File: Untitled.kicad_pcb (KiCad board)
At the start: 2 copper layers, 111.8 x 37.5 mm, 28 parts, among them J1 JAMMA, J2 CONN_01X06, J5 PWR_IN, J6 DC2DC, J7 SCART-F, SW1 SW_Push, SW2 SW_Push, SW3 SW_Push, U1 LD1117S33TR, U2 ESP32-WROOM, U3 TLC5926IDW, U4 TLC5926IDW

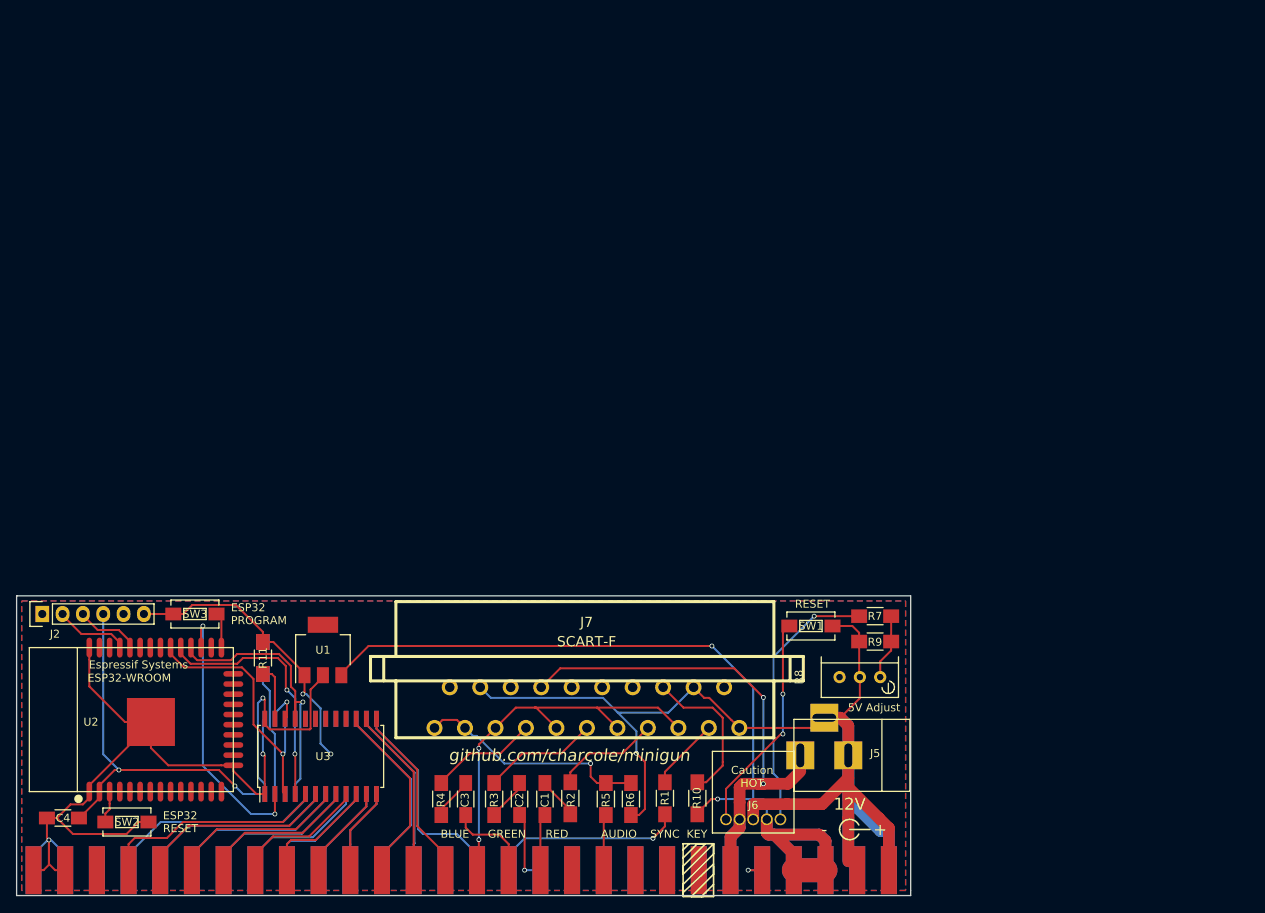
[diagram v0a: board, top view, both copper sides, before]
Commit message: Lynn almost done
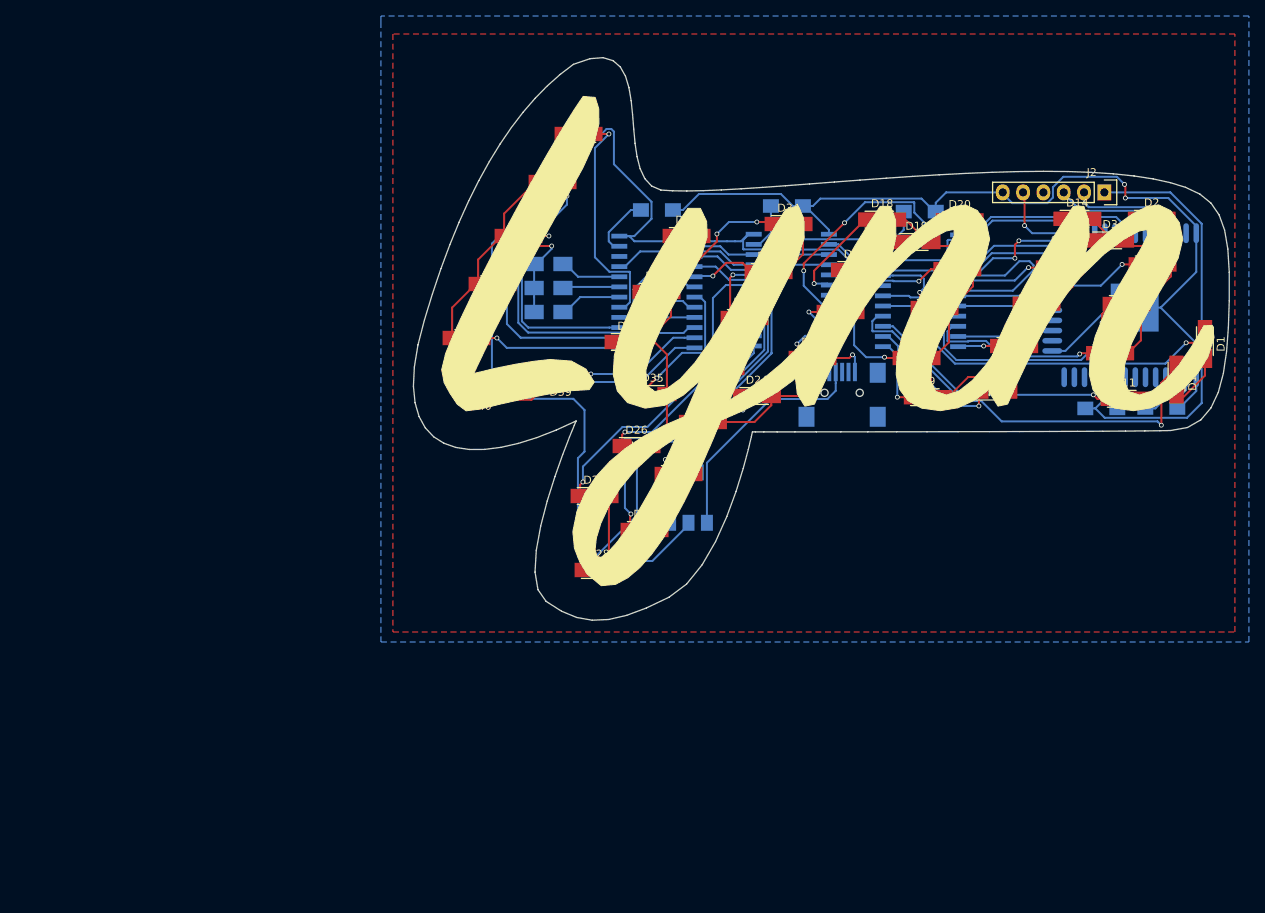
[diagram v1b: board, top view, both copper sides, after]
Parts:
- removed C1, C2, C3: 4.7u, Capacitors_SMD:C_1206_HandSoldering
- removed J5: PWR_IN, Connectors:BARREL_JACK
- removed J6: DC2DC, NQR010A0X4Z:NQR010A0X4Z
- removed J7: SCART-F, w_conn_av:SCART
- removed R10: 100, Resistors_SMD:R_1206_HandSoldering
- removed R3, R4: 330, Resistors_SMD:R_1206_HandSoldering
- removed R5: 10K, Resistors_SMD:R_1206_HandSoldering
- removed R6: 1K, Resistors_SMD:R_1206_HandSoldering
- removed R7: 240, Resistors_SMD:R_1206_HandSoldering
- removed R8: 500, Potentiometers:Potentiometer_Bourns_3296W_3-8Zoll_Inline_ScrewUp
- removed R9: 33, Resistors_SMD:R_1206_HandSoldering
- removed SW1, SW2, SW3: SW_Push, Buttons_Switches_SMD:SW_SPST_EVQPE1
- added D1: LED, LEDs:LED_1206_HandSoldering, F.Cu at (241.2, 94.2)
- added D10: LED, LEDs:LED_1206_HandSoldering, F.Cu at (214.8, 100.2)
- added D11: LED, LEDs:LED_1206_HandSoldering, F.Cu at (231.2, 101.1)
- added D12: LED, LEDs:LED_1206_HandSoldering, F.Cu at (237.7, 98.7)
- added D13: LED, LEDs:LED_1206_HandSoldering, F.Cu at (223.1, 84.7)
- added D14: LED, LEDs:LED_1206_HandSoldering, F.Cu at (225.3, 78.6)
- added D15: LED, LEDs:LED_1206_HandSoldering, F.Cu at (205.2, 96.0)
- added D16: LED, LEDs:LED_1206_HandSoldering, F.Cu at (207.4, 89.8)
- added D17: LED, LEDs:LED_1206_HandSoldering, F.Cu at (197.5, 85.0)
- added D18: LED, LEDs:LED_1206_HandSoldering, F.Cu at (200.9, 78.7)
- added D19: LED, LEDs:LED_1206_HandSoldering, F.Cu at (205.2, 81.5)
- added D2: LED, LEDs:LED_1206_HandSoldering, F.Cu at (234.6, 78.6)
- added D20: LED, LEDs:LED_1206_HandSoldering, F.Cu at (210.6, 78.8)
- added D21: LED, LEDs:LED_1206_HandSoldering, F.Cu at (210.3, 84.9)
- added D22: LED, LEDs:LED_1206_HandSoldering, F.Cu at (195.7, 90.2)
- added D23: LED, LEDs:LED_1206_HandSoldering, F.Cu at (192.2, 96.0)
- added D24: LED, LEDs:LED_1206_HandSoldering, F.Cu at (185.2, 100.8)
- added D25: LED, LEDs:LED_1206_HandSoldering, F.Cu at (178.5, 104.0)
- added D26: LED, LEDs:LED_1206_HandSoldering, F.Cu at (170.2, 107.0)
- added D27: LED, LEDs:LED_1206_HandSoldering, F.Cu at (164.9, 113.2)
- added D28: LED, LEDs:LED_1206_HandSoldering, F.Cu at (165.4, 122.5)
- added D29: LED, LEDs:LED_1206_HandSoldering, F.Cu at (171.2, 117.5)
- added D3: LED, LEDs:LED_1206_HandSoldering, F.Cu at (229.4, 81.3)
- added D30: LED, LEDs:LED_1206_HandSoldering, F.Cu at (175.4, 110.5)
- added D31: LED, LEDs:LED_1206_HandSoldering, F.Cu at (180.7, 97.2)
- added D32: LED, LEDs:LED_1206_HandSoldering, F.Cu at (183.7, 91.0)
- added D33: LED, LEDs:LED_1206_HandSoldering, F.Cu at (186.7, 85.2)
- added D34: LED, LEDs:LED_1206_HandSoldering, F.Cu at (189.2, 79.2)
- added D35: LED, LEDs:LED_1206_HandSoldering, F.Cu at (172.2, 100.5)
- added D36: LED, LEDs:LED_1206_HandSoldering, F.Cu at (169.2, 94.0)
- added D37: LED, LEDs:LED_1206_HandSoldering, F.Cu at (172.7, 87.8)
- added D38: LED, LEDs:LED_1206_HandSoldering, F.Cu at (176.4, 80.8)
- added D39: LED, LEDs:LED_1206_HandSoldering, F.Cu at (160.7, 98.2)
- added D4: LED, LEDs:LED_1206_HandSoldering, F.Cu at (234.7, 84.3)
- added D40: LED, LEDs:LED_1206_HandSoldering, F.Cu at (150.7, 100.0)
- added D41: LED, LEDs:LED_1206_HandSoldering, F.Cu at (148.9, 93.5)
- added D42: LED, LEDs:LED_1206_HandSoldering, F.Cu at (152.2, 86.8)
- added D43: LED, LEDs:LED_1206_HandSoldering, F.Cu at (155.4, 80.8)
- added D44: LED, LEDs:LED_1206_HandSoldering, F.Cu at (159.7, 74.0)
- added D45: LED, LEDs:LED_1206_HandSoldering, F.Cu at (162.9, 68.0)
- added D46: LED, LEDs:LED_1206_HandSoldering, B.Cu at (159.2, 90.2)
- added D47: LED, LEDs:LED_1206_HandSoldering, B.Cu at (159.2, 87.2)
- added D48: LED, LEDs:LED_1206_HandSoldering, B.Cu at (159.2, 84.2)
- added D5: LED, LEDs:LED_1206_HandSoldering, F.Cu at (231.4, 89.2)
- added D6: LED, LEDs:LED_1206_HandSoldering, F.Cu at (229.4, 95.4)
- added D7: LED, LEDs:LED_1206_HandSoldering, F.Cu at (220.2, 89.2)
- added D8: LED, LEDs:LED_1206_HandSoldering, F.Cu at (217.4, 94.5)
- added D9: LED, LEDs:LED_1206_HandSoldering, F.Cu at (206.6, 100.9)
- added U5: TLC5926IDW, Housings_SOIC:SOIC-24W_7.5x15.4mm_Pitch1.27mm, B.Cu at (172.8, 87.8)
- added lynn_outline: G***, svg2mod:lynn_outline, F.Cu at (175.0, 85.2)
- C4, R2, U1, U2, U3: moved to B.Cu
- J1: value JAMMA -> USB_B; footprint JAMMA:JAMMA -> Connectors:USB_Mini-B; moved to B.Cu
- R1: value 330 -> 10K; moved to B.Cu
- R11: value R -> 330; moved to B.Cu
- R12: value R -> 330
- moved C4 146.5 mm to (235.8, 102.3), turned to 0 degrees
- moved J2 142.8 mm to (228.7, 75.3), turned to 270 degrees
- moved U2 138.0 mm to (234.9, 89.4)
- moved R11 99.3 mm to (205.6, 77.7), turned to 0 degrees
- moved U3 94.9 mm to (205.7, 87.6), turned to 180 degrees
- moved R12 86.5 mm to (189.0, 77.0), turned to 0 degrees
- moved U4 82.8 mm to (189.6, 87.5), turned to 180 degrees
- moved J1 77.4 mm to (195.9, 101.2), turned to 90 degrees
- moved R2 74.3 mm to (172.8, 77.5), turned to 0 degrees
- moved R1 73.1 mm to (228.3, 102.3), turned to 180 degrees
- moved U1 49.5 mm to (176.7, 113.5)
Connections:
- J1 pad 1: GND -> +5V
- J1 pad 2: GND -> (no net)
- J1 pad 3: GND -> (no net)
- J1 pad 5: +5V -> (no net)
- J1 pad 6: +5V -> (no net)
- J2 pad 1: (no net) -> RESET
- J2 pad 5: (no net) -> PROG
- R1 pad 1: Net-(J7-Pad19) -> 33
- R1 pad 2: SYNC -> RESET
- R2 pad 2: Net-(C1-Pad2) -> GND
- U2 pad 25: Net-(SW3-Pad1) -> PROG
- U2 pad 29: LATCH -> (no net)
- U2 pad 3: Net-(SW2-Pad2) -> RESET
- U2 pad 30: CLK -> LATCH
- U2 pad 31: (no net) -> CLK
- U3 pad 10: LEFT1 -> Net-(D6-Pad1)
- U3 pad 11: DOWN1 -> Net-(D7-Pad1)
- U3 pad 12: UP1 -> Net-(D8-Pad1)
- U3 pad 13: TEST -> Net-(D9-Pad1)
- U3 pad 14: COIN1 -> Net-(D10-Pad1)
- U3 pad 15: START1 -> Net-(D11-Pad1)
- U3 pad 16: (no net) -> Net-(D12-Pad1)
- U3 pad 17: (no net) -> Net-(D13-Pad1)
- U3 pad 18: (no net) -> Net-(D14-Pad1)
- U3 pad 19: (no net) -> Net-(D15-Pad1)
- U3 pad 20: (no net) -> Net-(D16-Pad1)
- U3 pad 5: D1 -> Net-(D1-Pad1)
- U3 pad 6: C1 -> Net-(D2-Pad1)
- U3 pad 7: B1 -> Net-(D3-Pad1)
- U3 pad 8: A1 -> Net-(D4-Pad1)
- U3 pad 9: RIGHT1 -> Net-(D5-Pad1)
- U4 pad 10: START2 -> Net-(D22-Pad1)
- U4 pad 11: COIN2 -> Net-(D23-Pad1)
- U4 pad 12: SERVICE -> Net-(D24-Pad1)
- U4 pad 13: UP2 -> Net-(D25-Pad1)
- U4 pad 14: DOWN2 -> Net-(D26-Pad1)
- U4 pad 15: LEFT2 -> Net-(D27-Pad1)
- U4 pad 16: RIGHT2 -> Net-(D28-Pad1)
- U4 pad 17: A2 -> Net-(D29-Pad1)
- U4 pad 18: B2 -> Net-(D30-Pad1)
- U4 pad 19: C2 -> Net-(D31-Pad1)
- U4 pad 20: D2 -> Net-(D32-Pad1)
- U4 pad 22: (no net) -> Net-(U4-Pad22)
- U4 pad 5: (no net) -> Net-(D17-Pad1)
- U4 pad 6: (no net) -> Net-(D18-Pad1)
- U4 pad 7: (no net) -> Net-(D19-Pad1)
- U4 pad 8: (no net) -> Net-(D20-Pad1)
- U4 pad 9: (no net) -> Net-(D21-Pad1)
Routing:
- net +5V: track 126.2 -> 331.6 mm, vias 2 -> 3
- net GND: track 312.1 -> 162.7 mm, vias 5 -> 2
- net 33: track 77.8 -> 153.4 mm, vias 3 -> 0
- net +12V: track 69.1 -> 0.00 mm, vias 2 -> 0
- net Net-(D1-Pad1): track 0.00 -> 67.3 mm, vias 0 -> 1
- net RESET: track 0.00 -> 64.2 mm
- net Net-(D12-Pad1): track 0.00 -> 53.3 mm, vias 0 -> 1
- net VIDEO_GND: track 51.1 -> 0.00 mm, vias 2 -> 0
- net Net-(D28-Pad1): track 0.00 -> 45.3 mm, vias 0 -> 1
- net Net-(D29-Pad1): track 0.00 -> 43.7 mm, vias 0 -> 1
- net Net-(D44-Pad1): track 0.00 -> 37.4 mm, vias 0 -> 1
- net Net-(J6-Pad5): track 33.5 -> 0.00 mm, vias 1 -> 0
- net Net-(D11-Pad1): track 0.00 -> 32.9 mm, vias 0 -> 1
- net Net-(D27-Pad1): track 0.00 -> 32.5 mm, vias 0 -> 1
- net Net-(D5-Pad1): track 0.00 -> 31.5 mm, vias 0 -> 1
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- added copper zone on F.Cu, net +5V
- removed copper zone on F.Cu, net GND
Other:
- board size 111.8 x 37.5 mm -> 102 x 70.3 mm
- board text removed: "+"
- board text removed: "-"
- board text removed: "12V"
- board text removed: "5V Adjust"
- board text removed: "AUDIO"
- board text removed: "BLUE"
- board text removed: "Caution HOT"
- board text removed: "ESP32 PROGRAM"
- board text removed: "ESP32 RESET"
- board text removed: "GREEN"
- board text removed: "KEY"
- board text removed: "RED"
- board text removed: "RESET"
- board text removed: "SYNC"
- board text removed: "github.com/charcole/minigun"
